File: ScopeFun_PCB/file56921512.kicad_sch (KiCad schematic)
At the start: 33 parts, among them IC1 AD9643BCPZ-250, U11 LTC6957-2, U9 SG3225VAN-250Mhz

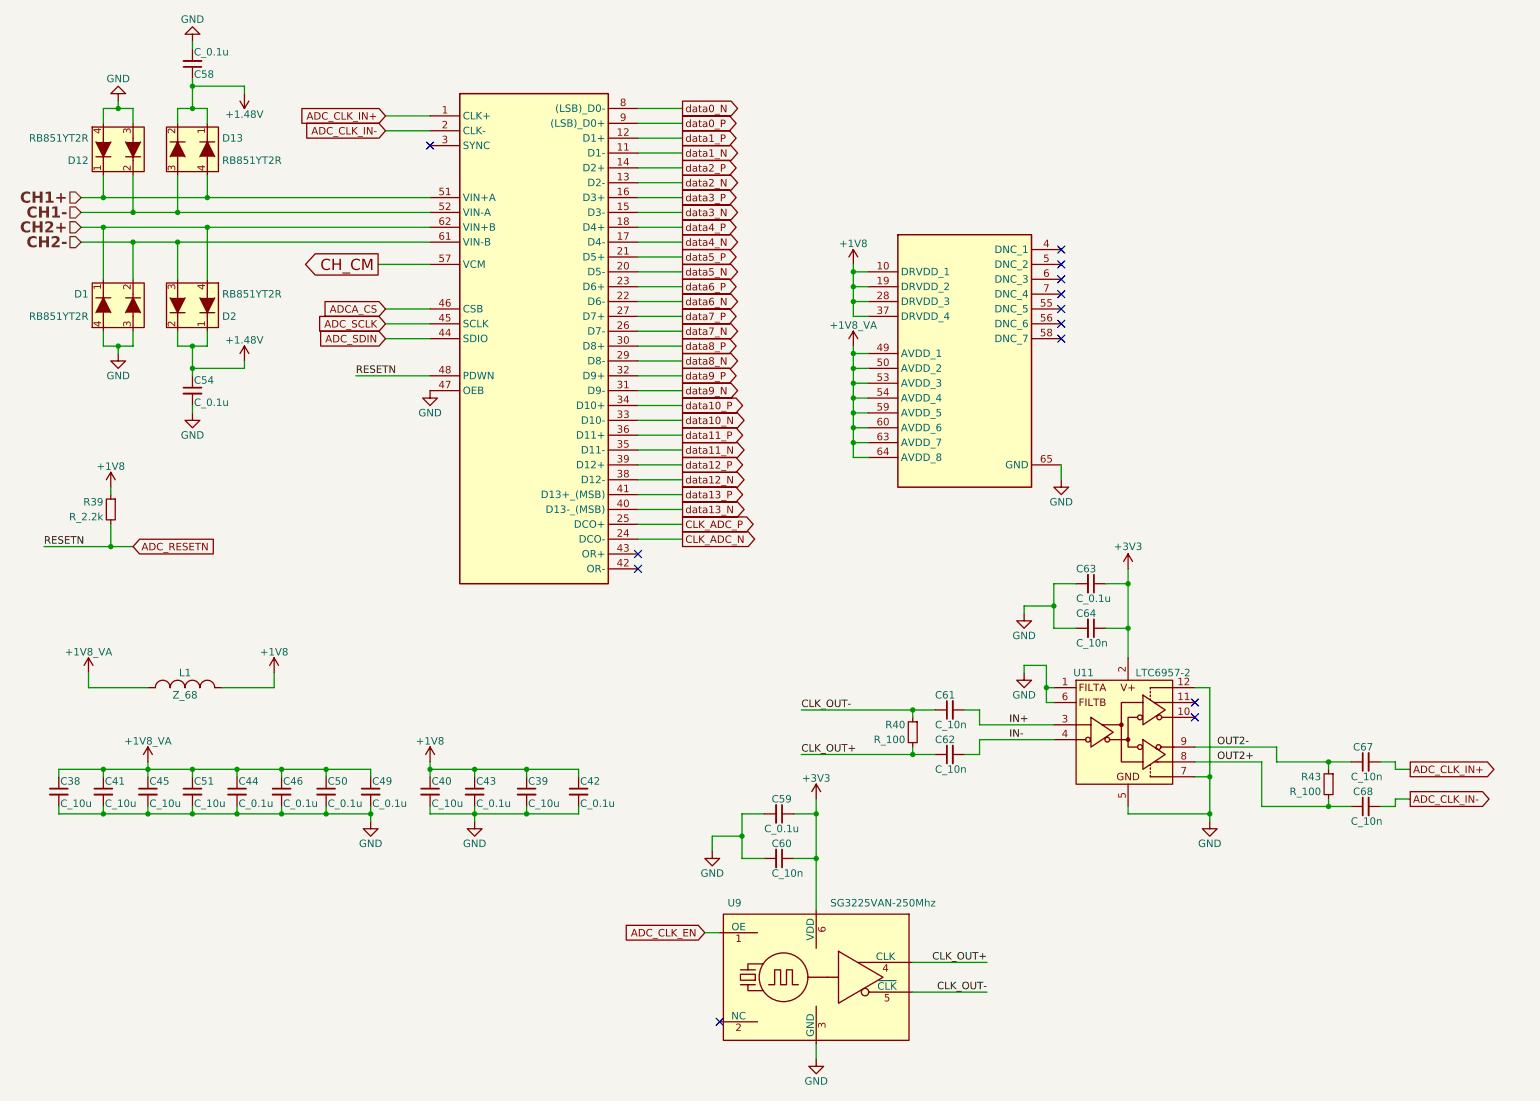
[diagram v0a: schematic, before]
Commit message: 260417_diff_comp
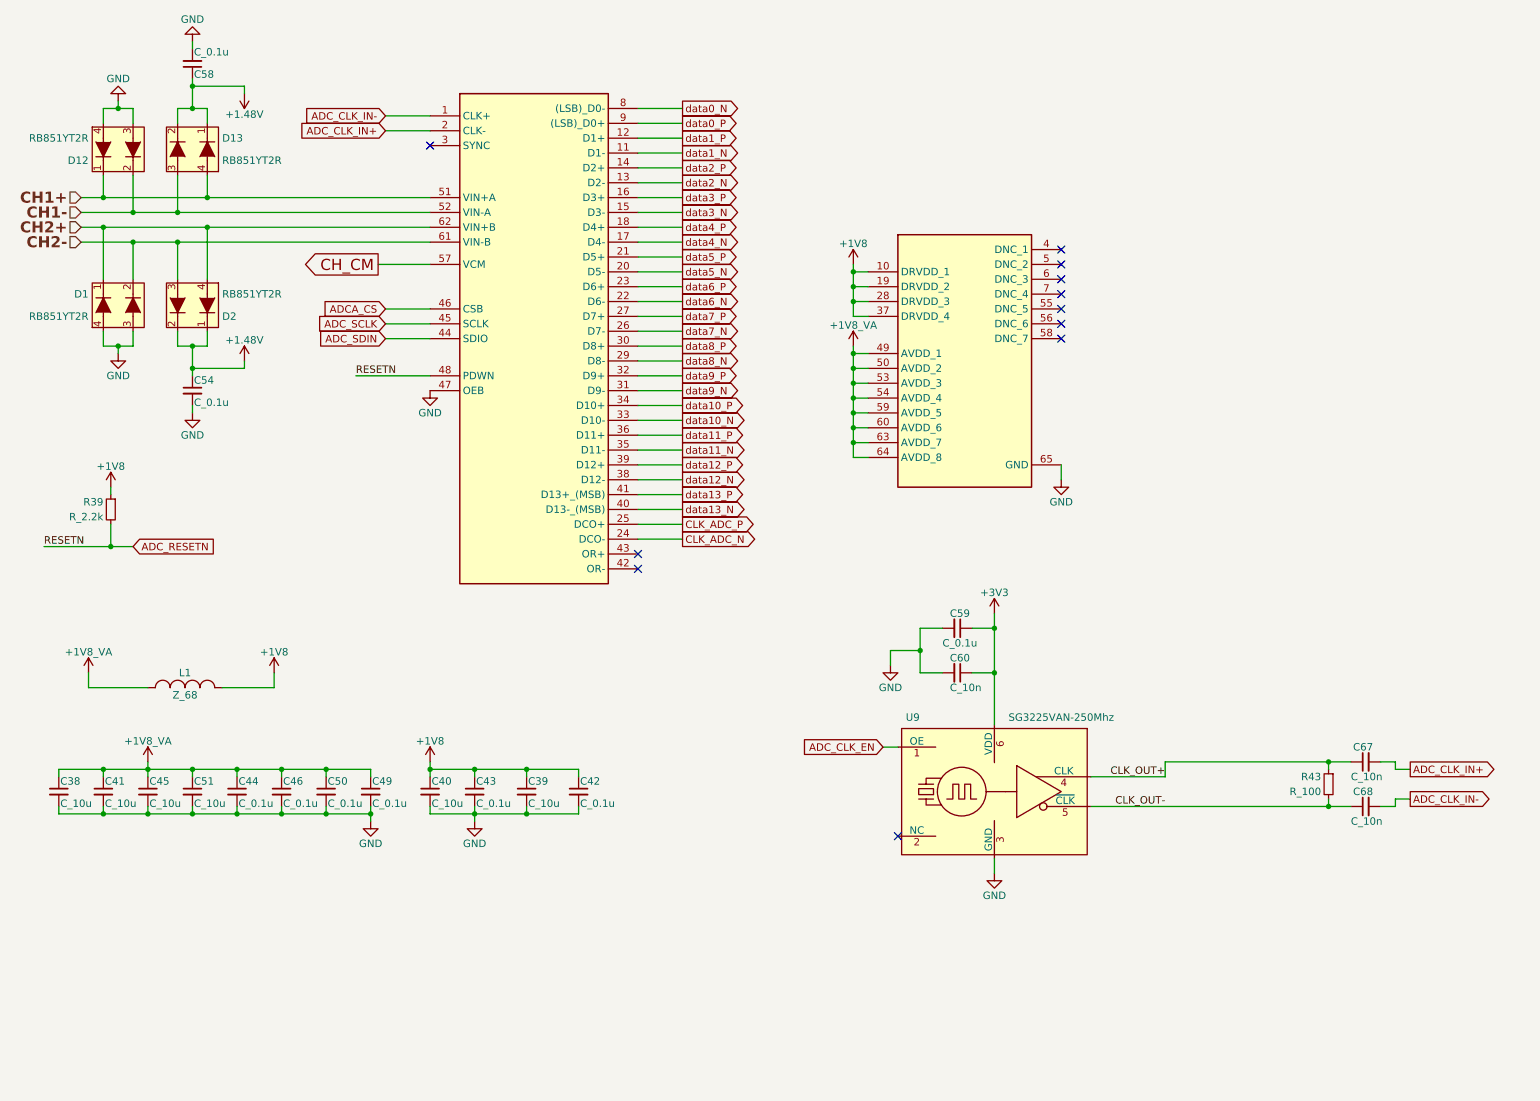
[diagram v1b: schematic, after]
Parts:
- removed C61, C62, C64: C_10n, ScopefunPackagesLibrary:C_0402, symbol ScopefunParts:C_10n_0402
- removed C63: C_0.1u, ScopefunPackagesLibrary:C_0603, symbol ScopefunParts:C_0.1u
- removed R40: R_100, ScopefunPackagesLibrary:R_0402, symbol ScopefunParts:R_100
- removed U11: LTC6957-2, ScopefunPackagesLibrary:12-MSOP, symbol ScopefunParts:LTC6957-2
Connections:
- net OUT2+ is gone; now on net CLK_OUT-: C68.1, R43.2
- net OUT2- is gone; now on net CLK_OUT+: C67.1, R43.1
- net ADC_CLK_IN+: now also IC1.2 (CLK-); no longer IC1.1 (CLK+)
- net ADC_CLK_IN-: now also IC1.1 (CLK+); no longer IC1.2 (CLK-)
- no-connect marks 13 -> 11
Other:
- moved on the sheet: C59, C60, U9

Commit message: 260420
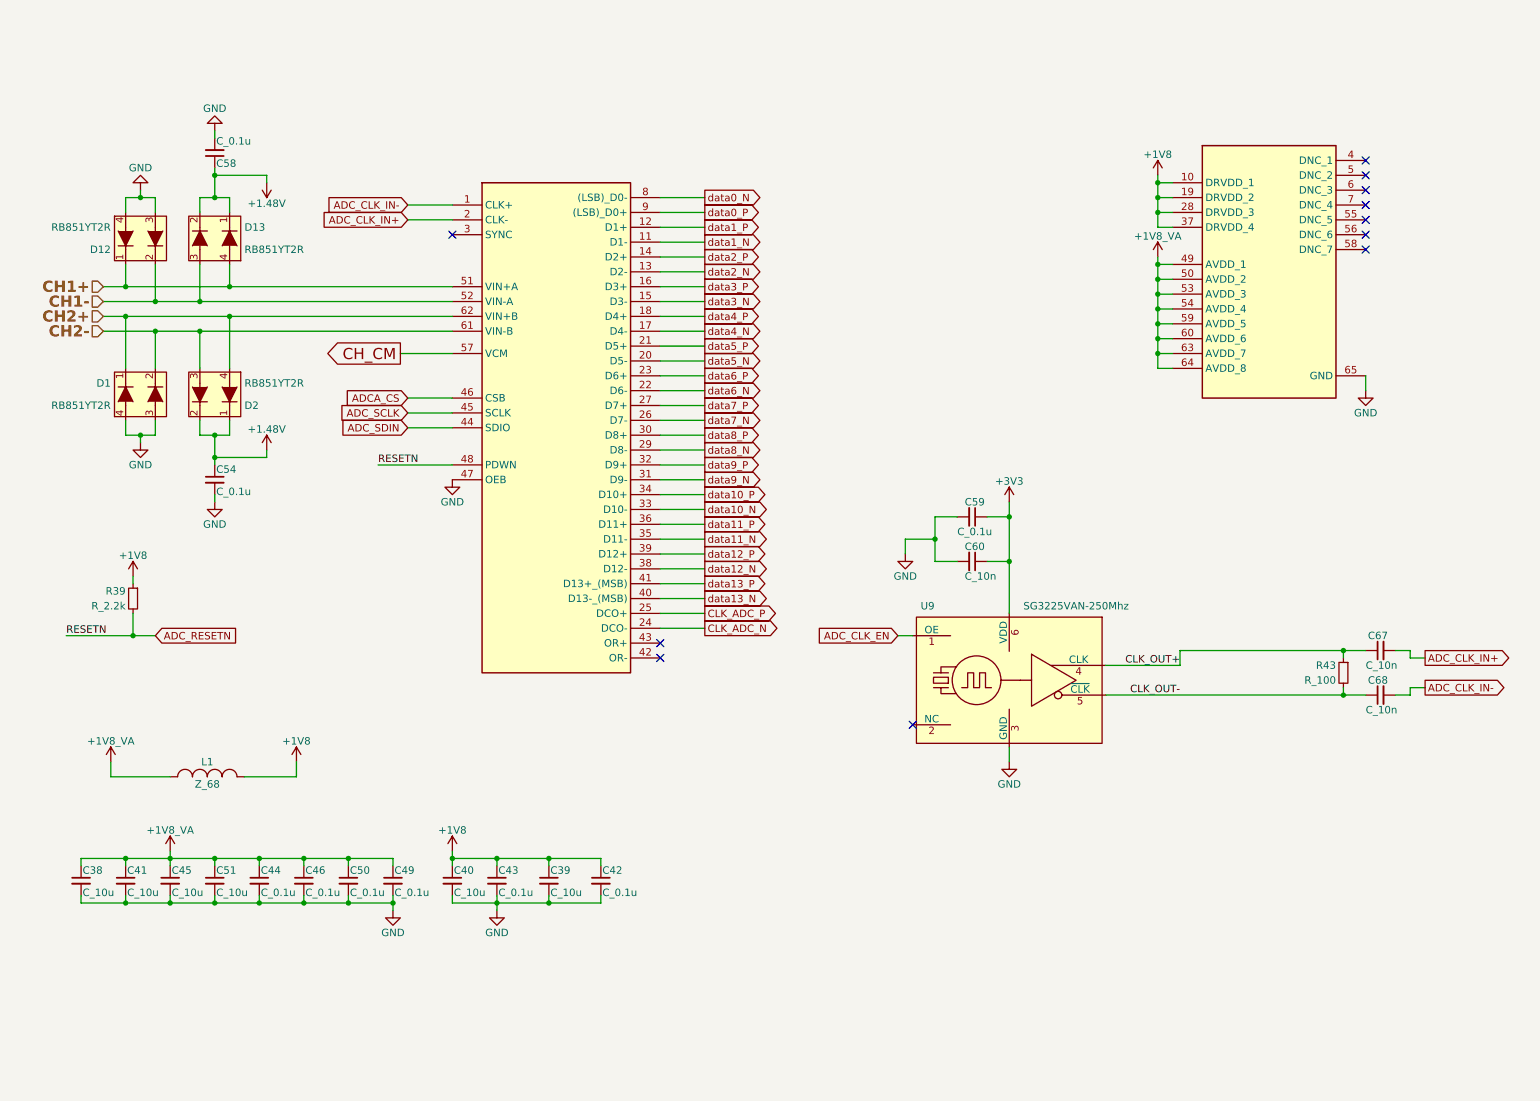
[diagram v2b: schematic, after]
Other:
- moved on the sheet: C38, C39, C40, C41, C42, C43, C44, C45, C46, C49, C50, C51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
